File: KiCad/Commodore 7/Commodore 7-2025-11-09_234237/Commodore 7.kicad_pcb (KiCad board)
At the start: 2 copper layers, 41 parts, among them IC1 BGU7004,115, J1 M20-6112045, U1 TMP112AIDRLR-Temperature, U10 TCA9543APWR, U2 NEO-M9N-00B, U3 BMI270 - Secondary Accelerome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, U4 MMC5983MA-Magnetomer, U5 MS560702BA03-50 - Barometer, U6 TCA9509DGKR, U7 SN65HVD74DR, U8 IIM-42652 - Main Acceleromete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, U9 IIM-42652 Main Accelerometer

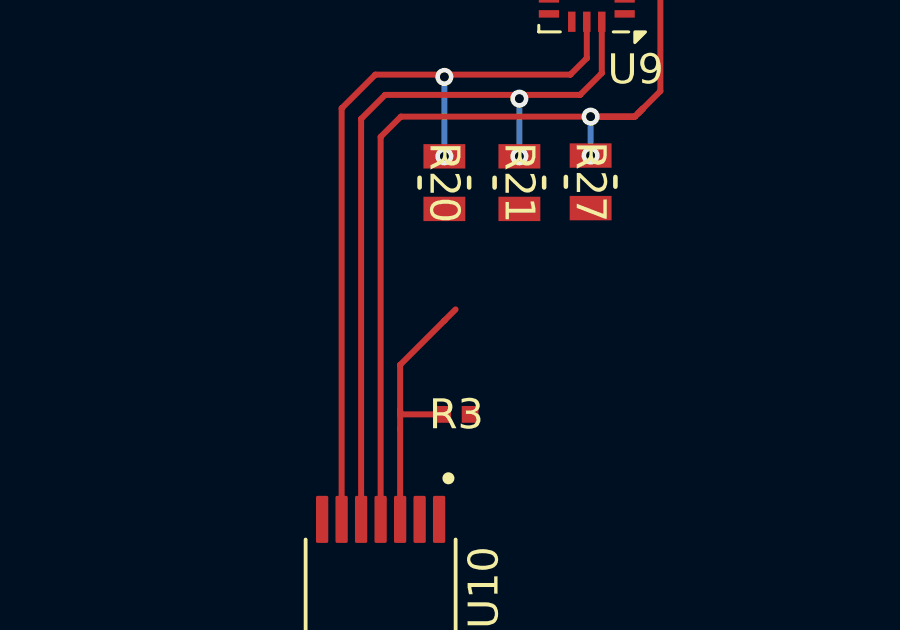
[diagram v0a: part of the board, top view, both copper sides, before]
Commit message: updated some labels idk
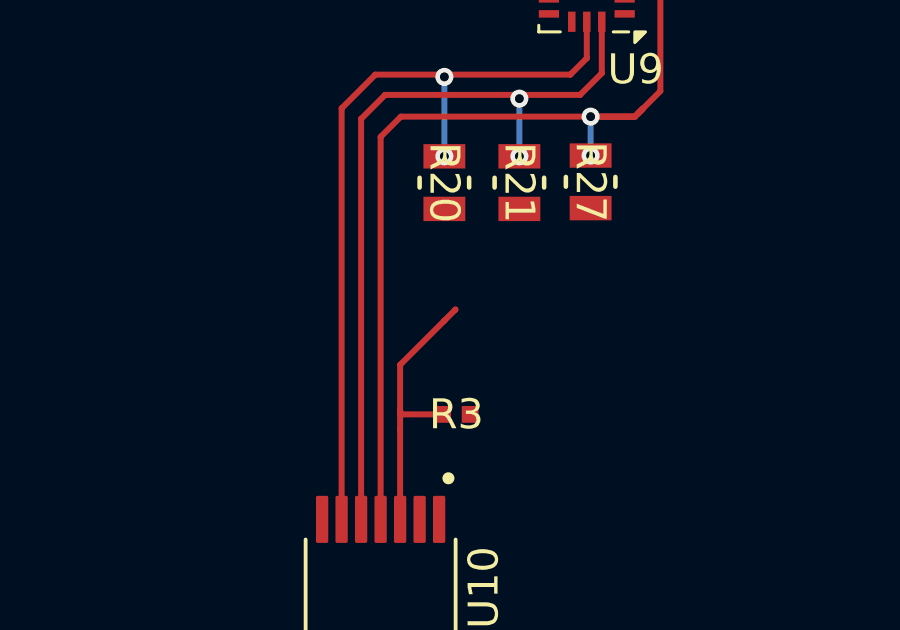
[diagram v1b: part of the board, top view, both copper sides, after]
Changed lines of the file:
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@@
+	)
+	(segment
+		(start 131.085 88.915)
+		(end 131.1 88.9)
+		(width 0.2)
+		(layer "F.Cu")
+		(net 45)
 	)
 	(segment
@@
 	(segment
 		(start 130.725 89.275)
-		(end 131.1 88.9)
+		(end 131.085 88.915)
 		(width 0.2)
 		(layer "F.Cu")
